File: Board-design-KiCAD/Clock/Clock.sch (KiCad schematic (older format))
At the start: 19 parts, among them M1 SevSeg4Inch, M2 SevSeg4Inch, Y1 SevSeg1.8Inch, Y2 SevSeg1.8Inch, Y3 SevSeg1.8Inch, Y4 SevSeg1.8Inch

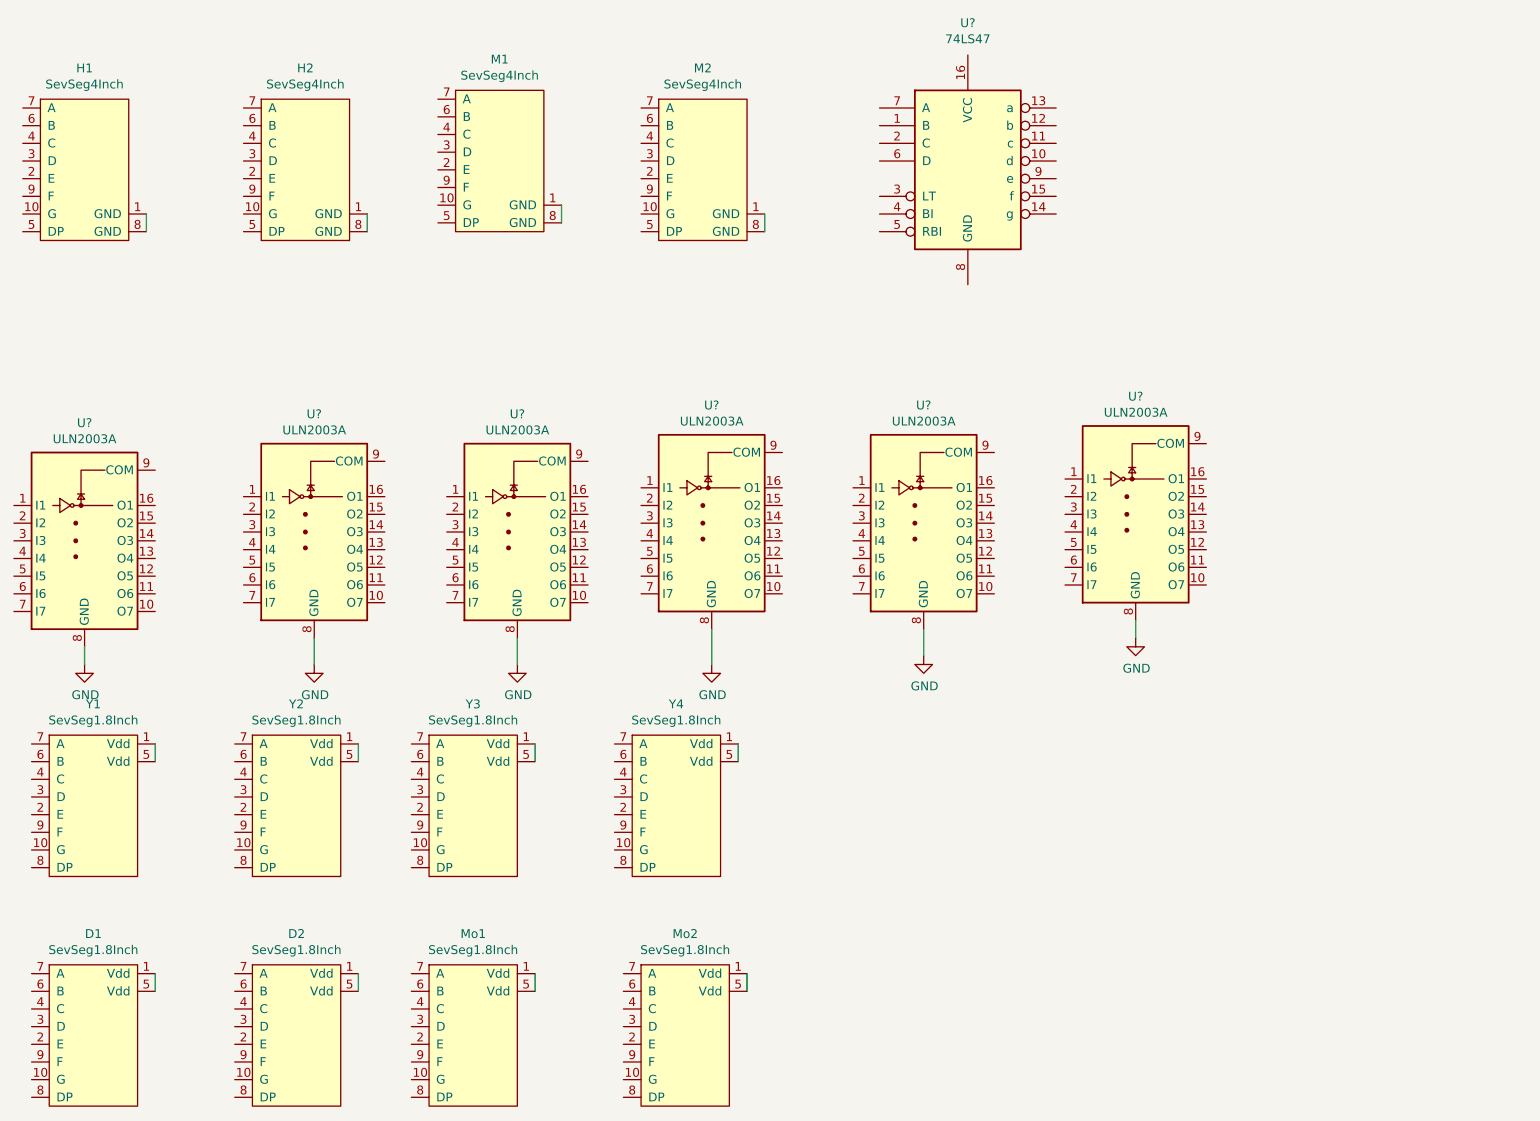
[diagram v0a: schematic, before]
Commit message: Add some components
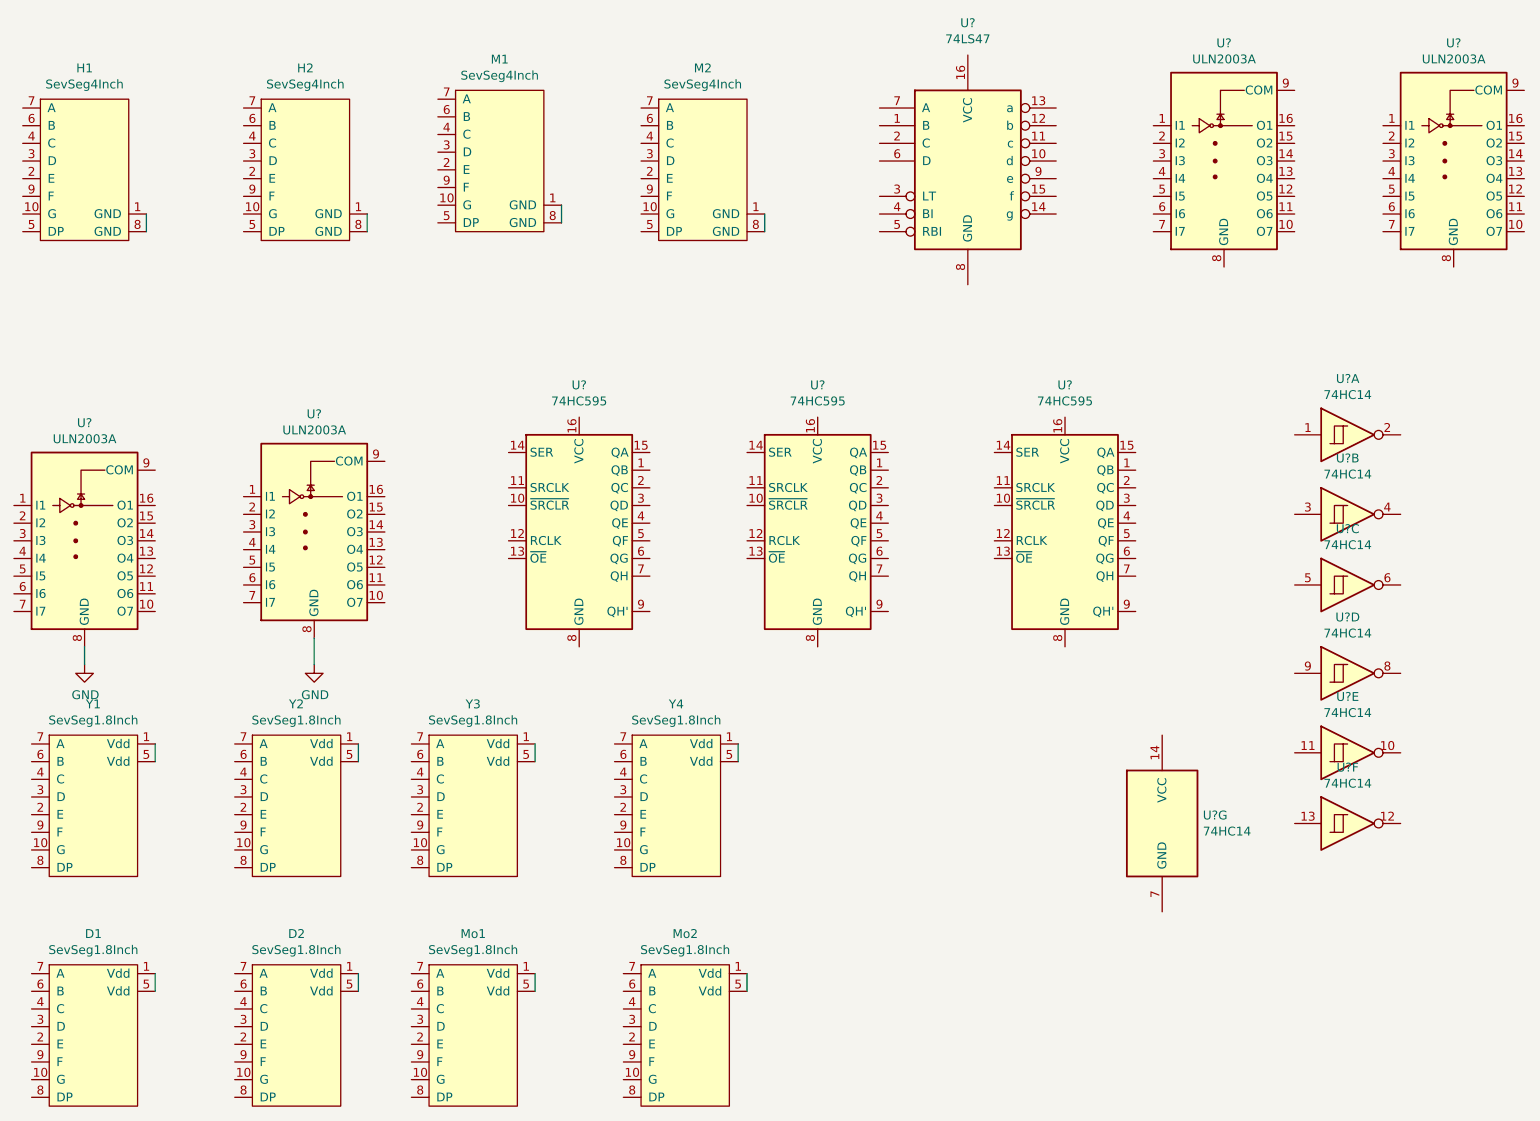
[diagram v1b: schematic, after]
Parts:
- removed U? (x4): ULN2003A, symbol Transistor_Array:ULN2003A
- added U? (x3): 74HC595, symbol 74xx:74HC595
- added U? (x2): ULN2003A, symbol Transistor_Array:ULN2003A
- added U? (x7): 74HC14, symbol 74xx:74HC14
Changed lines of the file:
@@
-$EndComp
-$Comp
-L Transistor_Array:ULN2003A U?
-U 1 1 5F3B85A2
-P 4450 3800
-F 0 "U?" H 4450 4467 50  0000 C CNN
-F 1 "ULN2003A" H 4450 4376 50  0000 C CNN
-F 2 "" H 4500 3250 50  0001 L CNN
-F 3 "http://www.ti.com/lit/ds/symlink/uln2003a.pdf" H 4550 3600 50  0001 C CNN
-	1    4450 3800
-	1    0    0    -1
-$EndComp
-$Comp
-L Transistor_Array:ULN2003A U?
-U 1 1 5F3B9616
-P 5550 3750
-F 0 "U?" H 5550 4417 50  0000 C CNN
-F 1 "ULN2003A" H 5550 4326 50  0000 C CNN
-F 2 "" H 5600 3200 50  0001 L CNN
-F 3 "http://www.ti.com/lit/ds/symlink/uln2003a.pdf" H 5650 3550 50  0001 C CNN
-	1    5550 3750
-	1    0    0    -1
-$EndComp
-$Comp
-L Transistor_Array:ULN2003A U?
-U 1 1 5F3BAC84
-P 6750 3750
-F 0 "U?" H 6750 4417 50  0000 C CNN
-F 1 "ULN2003A" H 6750 4326 50  0000 C CNN
-F 2 "" H 6800 3200 50  0001 L CNN
-F 3 "http://www.ti.com/lit/ds/symlink/uln2003a.pdf" H 6850 3550 50  0001 C CNN
-	1    6750 3750
-	1    0    0    -1
-$EndComp
-$Comp
-L Transistor_Array:ULN2003A U?
-U 1 1 5F3BBFEA
-P 7950 3700
-F 0 "U?" H 7950 4367 50  0000 C CNN
-F 1 "ULN2003A" H 7950 4276 50  0000 C CNN
-F 2 "" H 8000 3150 50  0001 L CNN
-F 3 "http://www.ti.com/lit/ds/symlink/uln2003a.pdf" H 8050 3500 50  0001 C CNN
-	1    7950 3700
-	1    0    0    -1
 $EndComp
 $Comp
@@
 	1    0    0    -1
 $EndComp
-$Comp
-L power:GND #PWR?
-U 1 1 5F3CCD46
-P 4450 4550
-F 0 "#PWR?" H 4450 4300 50  0001 C CNN
-F 1 "GND" H 4455 4377 50  0000 C CNN
-F 2 "" H 4450 4550 50  0001 C CNN
-F 3 "" H 4450 4550 50  0001 C CNN
-	1    4450 4550
-	1    0    0    -1
-$EndComp
-$Comp
-L power:GND #PWR?
-U 1 1 5F3CD13E
-P 5550 4550
-F 0 "#PWR?" H 5550 4300 50  0001 C CNN
-F 1 "GND" H 5555 4377 50  0000 C CNN
-F 2 "" H 5550 4550 50  0001 C CNN
-F 3 "" H 5550 4550 50  0001 C CNN
-	1    5550 4550
-	1    0    0    -1
-$EndComp
-$Comp
-L power:GND #PWR?
-U 1 1 5F3CD53D
-P 6750 4500
-F 0 "#PWR?" H 6750 4250 50  0001 C CNN
-F 1 "GND" H 6755 4327 50  0000 C CNN
-F 2 "" H 6750 4500 50  0001 C CNN
-F 3 "" H 6750 4500 50  0001 C CNN
-	1    6750 4500
-	1    0    0    -1
-$EndComp
-$Comp
-L power:GND #PWR?
-U 1 1 5F3CD948
-P 7950 4400
-F 0 "#PWR?" H 7950 4150 50  0001 C CNN
-F 1 "GND" H 7955 4227 50  0000 C CNN
-F 2 "" H 7950 4400 50  0001 C CNN
-F 3 "" H 7950 4400 50  0001 C CNN
-	1    7950 4400
-	1    0    0    -1
-$EndComp
 Wire Wire Line
 	2000 4450 2000 4550
 Wire Wire Line
 	3300 4400 3300 4550
-Wire Wire Line
-	4450 4400 4450 4550
-Wire Wire Line
-	5550 4350 5550 4550
-Wire Wire Line
-	6750 4350 6750 4500
-Wire Wire Line
-	7950 4300 7950 4400
 $Comp
 L Custom:SevSeg1.8Inch Y3
@@
 	1    0    0    -1
 $EndComp
+$Comp
+L 74xx:74HC595 U?
+U 1 1 5F61C67C
+P 4800 3750
+F 0 "U?" H 4800 4531 50  0000 C CNN
+F 1 "74HC595" H 4800 4440 50  0000 C CNN
+F 2 "" H 4800 3750 50  0001 C CNN
+F 3 "http://www.ti.com/lit/ds/symlink/sn74hc595.pdf" H 4800 3750 50  0001 C CNN
+	1    4800 3750
+	1    0    0    -1
+$EndComp
+$Comp
+L 74xx:74HC595 U?
+U 1 1 5F61CF1D
+P 6150 3750
+F 0 "U?" H 6150 4531 50  0000 C CNN
+F 1 "74HC595" H 6150 4440 50  0000 C CNN
+F 2 "" H 6150 3750 50  0001 C CNN
+F 3 "http://www.ti.com/lit/ds/symlink/sn74hc595.pdf" H 6150 3750 50  0001 C CNN
+	1    6150 3750
+	1    0    0    -1
+$EndComp
+$Comp
+L 74xx:74HC595 U?
+U 1 1 5F61DB6E
+P 7550 3750
+F 0 "U?" H 7550 4531 50  0000 C CNN
+F 1 "74HC595" H 7550 4440 50  0000 C CNN
+F 2 "" H 7550 3750 50  0001 C CNN
+F 3 "http://www.ti.com/lit/ds/symlink/sn74hc595.pdf" H 7550 3750 50  0001 C CNN
+	1    7550 3750
+	1    0    0    -1
+$EndComp
+$Comp
+L Transistor_Array:ULN2003A U?
+U 1 1 5F61F098
+P 8450 1700
+F 0 "U?" H 8450 2367 50  0000 C CNN
+F 1 "ULN2003A" H 8450 2276 50  0000 C CNN
+F 2 "" H 8500 1150 50  0001 L CNN
+F 3 "http://www.ti.com/lit/ds/symlink/uln2003a.pdf" H 8550 1500 50  0001 C CNN
+	1    8450 1700
+	1    0    0    -1
+$EndComp
+$Comp
+L Transistor_Array:ULN2003A U?
+U 1 1 5F6203B3
+P 9750 1700
+F 0 "U?" H 9750 2367 50  0000 C CNN
+F 1 "ULN2003A" H 9750 2276 50  0000 C CNN
+F 2 "" H 9800 1150 50  0001 L CNN
+F 3 "http://www.ti.com/lit/ds/symlink/uln2003a.pdf" H 9850 1500 50  0001 C CNN
+	1    9750 1700
+	1    0    0    -1
+$EndComp
+$Comp
+L 74xx:74HC14 U?
+U 1 1 5F621AF3
+P 9150 3250
+F 0 "U?" H 9150 3567 50  0000 C CNN
+F 1 "74HC14" H 9150 3476 50  0000 C CNN
+F 2 "" H 9150 3250 50  0001 C CNN
+F 3 "http://www.ti.com/lit/gpn/sn74HC14" H 9150 3250 50  0001 C CNN
+	1    9150 3250
+	1    0    0    -1
+$EndComp
+$Comp
+L 74xx:74HC14 U?
+U 2 1 5F623073
+P 9150 3700
+F 0 "U?" H 9150 4017 50  0000 C CNN
+F 1 "74HC14" H 9150 3926 50  0000 C CNN
+F 2 "" H 9150 3700 50  0001 C CNN
+F 3 "http://www.ti.com/lit/gpn/sn74HC14" H 9150 3700 50  0001 C CNN
+	2    9150 3700
+	1    0    0    -1
+$EndComp
+$Comp
+L 74xx:74HC14 U?
+U 3 1 5F62444F
+P 9150 4100
+F 0 "U?" H 9150 4417 50  0000 C CNN
+F 1 "74HC14" H 9150 4326 50  0000 C CNN
+F 2 "" H 9150 4100 50  0001 C CNN
+F 3 "http://www.ti.com/lit/gpn/sn74HC14" H 9150 4100 50  0001 C CNN
+	3    9150 4100
+	1    0    0    -1
+$EndComp
+$Comp
+L 74xx:74HC14 U?
+U 4 1 5F62485C
+P 9150 4600
+F 0 "U?" H 9150 4917 50  0000 C CNN
+F 1 "74HC14" H 9150 4826 50  0000 C CNN
+F 2 "" H 9150 4600 50  0001 C CNN
+F 3 "http://www.ti.com/lit/gpn/sn74HC14" H 9150 4600 50  0001 C CNN
+	4    9150 4600
+	1    0    0    -1
+$EndComp
+$Comp
+L 74xx:74HC14 U?
+U 5 1 5F625C4A
+P 9150 5050
+F 0 "U?" H 9150 5367 50  0000 C CNN
+F 1 "74HC14" H 9150 5276 50  0000 C CNN
+F 2 "" H 9150 5050 50  0001 C CNN
+F 3 "http://www.ti.com/lit/gpn/sn74HC14" H 9150 5050 50  0001 C CNN
+	5    9150 5050
+	1    0    0    -1
+$EndComp
+$Comp
+L 74xx:74HC14 U?
+U 6 1 5F627579
+P 9150 5450
+F 0 "U?" H 9150 5767 50  0000 C CNN
+F 1 "74HC14" H 9150 5676 50  0000 C CNN
+F 2 "" H 9150 5450 50  0001 C CNN
+F 3 "http://www.ti.com/lit/gpn/sn74HC14" H 9150 5450 50  0001 C CNN
+	6    9150 5450
+	1    0    0    -1
+$EndComp
+$Comp
+L 74xx:74HC14 U?
+U 7 1 5F62877C
+P 8100 5450
+F 0 "U?" H 8330 5496 50  0000 L CNN
+F 1 "74HC14" H 8330 5405 50  0000 L CNN
+F 2 "" H 8100 5450 50  0001 C CNN
+F 3 "http://www.ti.com/lit/gpn/sn74HC14" H 8100 5450 50  0001 C CNN
+	7    8100 5450
+	1    0    0    -1
+$EndComp
